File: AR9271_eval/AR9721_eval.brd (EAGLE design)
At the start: 160 x 100 mm, 125 parts, among them J1 UJ2-MIBH2-4-SMT-TR, J3 HTST-110-01-XX-DV, J7 132134-15, J8 132134-15, U1 U-ATHEROS-AR9271, U2 AT24C04C-XHM-T, U3 LT3080EQPBF, U4 LT3080EQPBF, U5 LT3080EQPBF, U6 LT3080EQPBF, Y1 ECS-400-10-36-CKY-TR

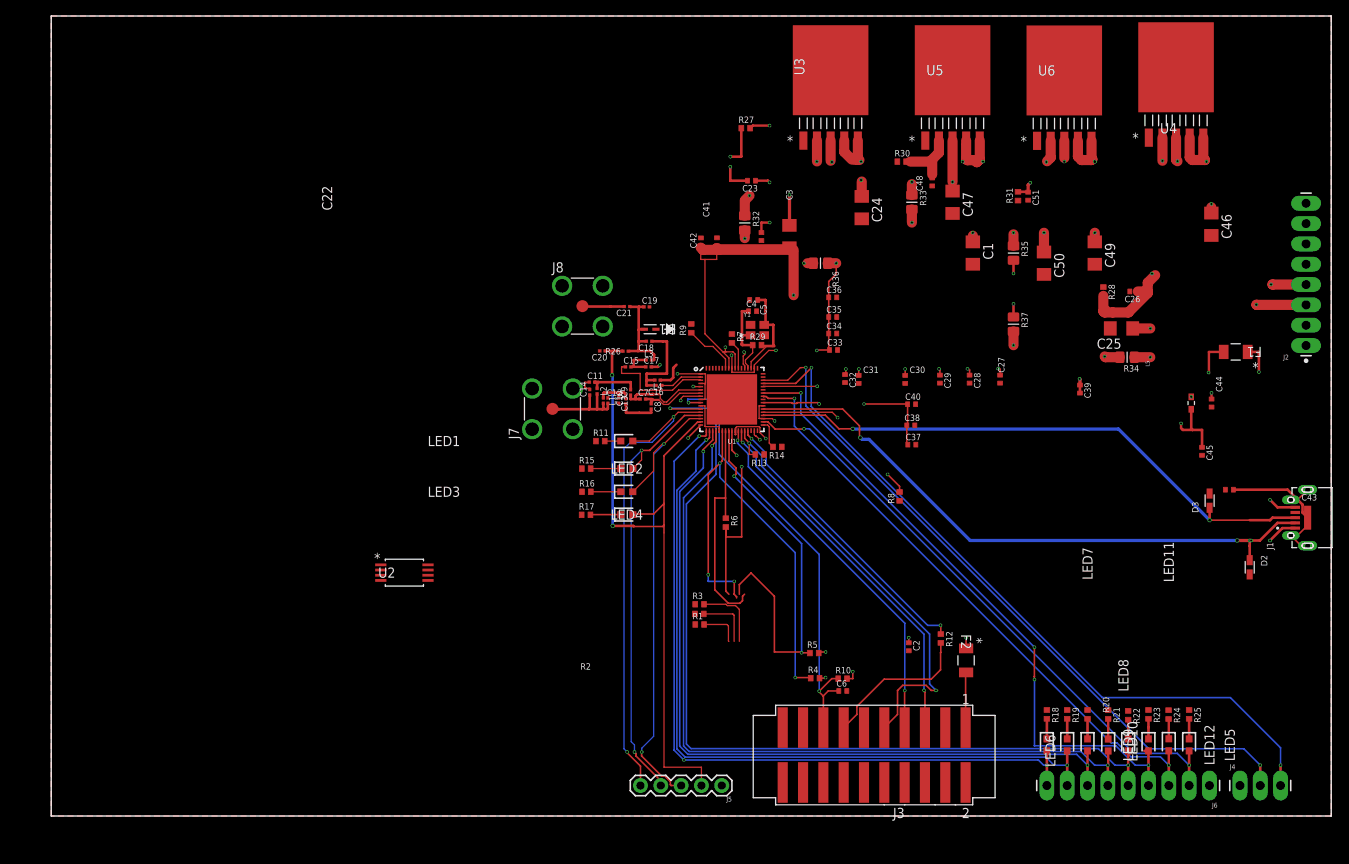
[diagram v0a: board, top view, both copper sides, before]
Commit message: Add files via upload
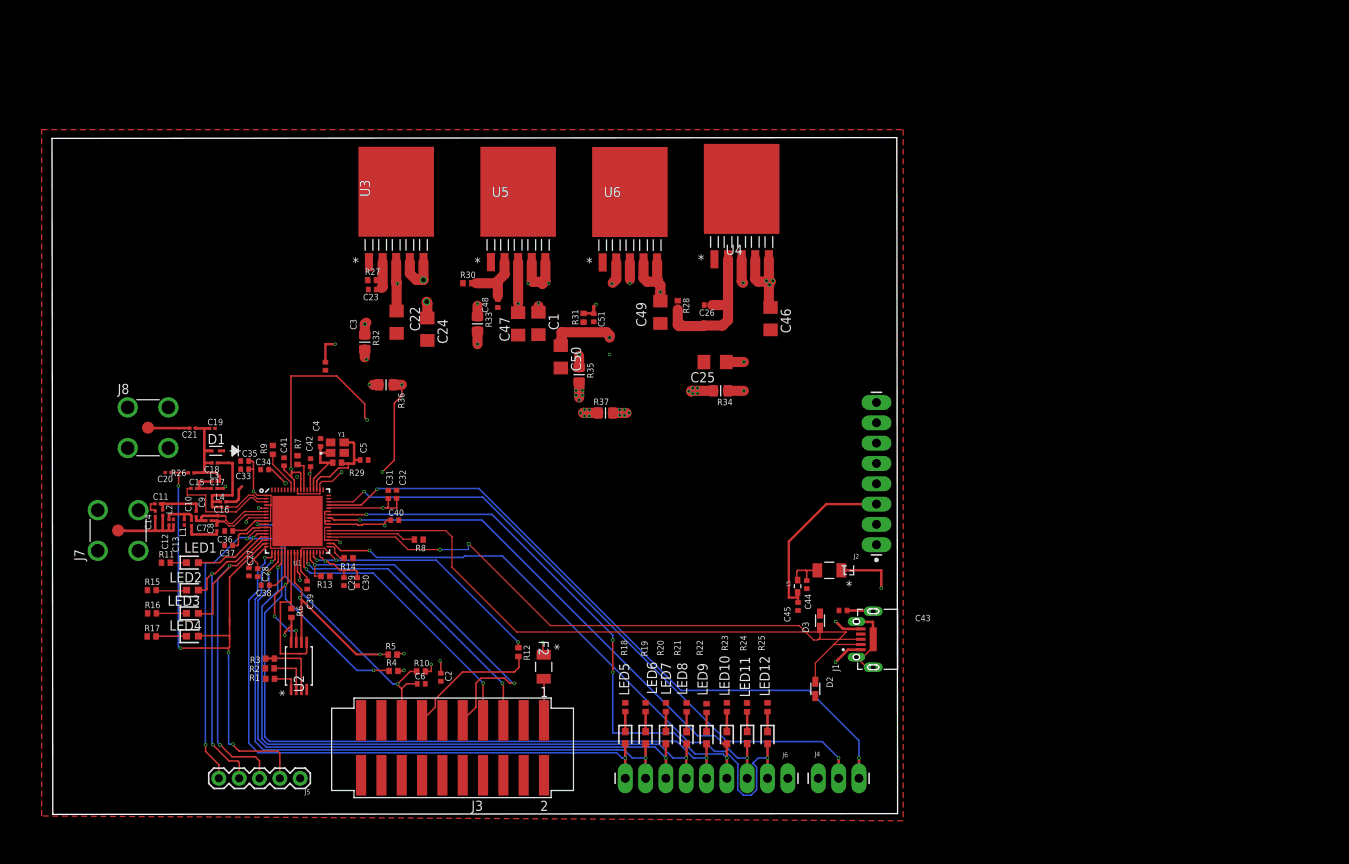
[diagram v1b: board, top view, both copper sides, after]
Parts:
- moved C39 99.7 mm to (32.0, 28.9)
- moved C27 96.9 mm to (24.7, 30.5)
- moved C28 92.2 mm to (25.8, 30.4)
- moved C37 86.3 mm to (22.2, 33.8), turned to 180 degrees
- moved C38 83.1 mm to (26.8, 28.8), turned to 180 degrees
- moved C36 80.9 mm to (22.2, 35.6), turned to 180 degrees
- moved C29 78.7 mm to (36.6, 29.3)
- moved C35 75.7 mm to (24.2, 44.4), turned to 180 degrees
- moved C33 75.1 mm to (24.2, 43.4), turned to 180 degrees
- moved C30 73.0 mm to (38.2, 29.3)
- moved C34 73.0 mm to (26.7, 43.3), turned to 180 degrees
- moved C40 66.2 mm to (43.0, 37.0)
- moved C50 61.5 mm to (63.7, 57.4)
- moved C41 60.7 mm to (29.1, 44.3)
- moved C31 60.5 mm to (42.1, 40.2), turned to 90 degrees
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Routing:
- net 3V3_D: track 202.7 -> 101.1 mm, vias 22 -> 15
- net LDO_IN: track 141.5 -> 90.0 mm, vias 11 -> 6
- net 1V2_A: track 91.9 -> 41.2 mm, vias 5 -> 3
- net N$25: track 53.2 -> 21.0 mm, vias 2 -> 0
- net N$3: track 57.8 -> 32.4 mm
- net GPIO11: track 114.3 -> 94.0 mm
- net N$23: track 23.2 -> 3.28 mm, vias 3 -> 0
- net RST_L: track 57.8 -> 41.0 mm
- net GPIO6: track 95.5 -> 78.8 mm
- net GPIO8: track 99.5 -> 82.7 mm
- net GPIO7: track 97.5 -> 80.7 mm
- net SWCOM1: track 55.9 -> 39.6 mm
- net GPIO5: track 93.7 -> 77.7 mm, vias 3 -> 2
- net SWCOM0: track 61.1 -> 45.1 mm
- net SWCOM2: track 60.7 -> 46.0 mm
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- removed copper zone on layer 15, net N$23
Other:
- board size 160 x 100 mm -> 105.7 x 84.6 mm

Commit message: Add files via upload
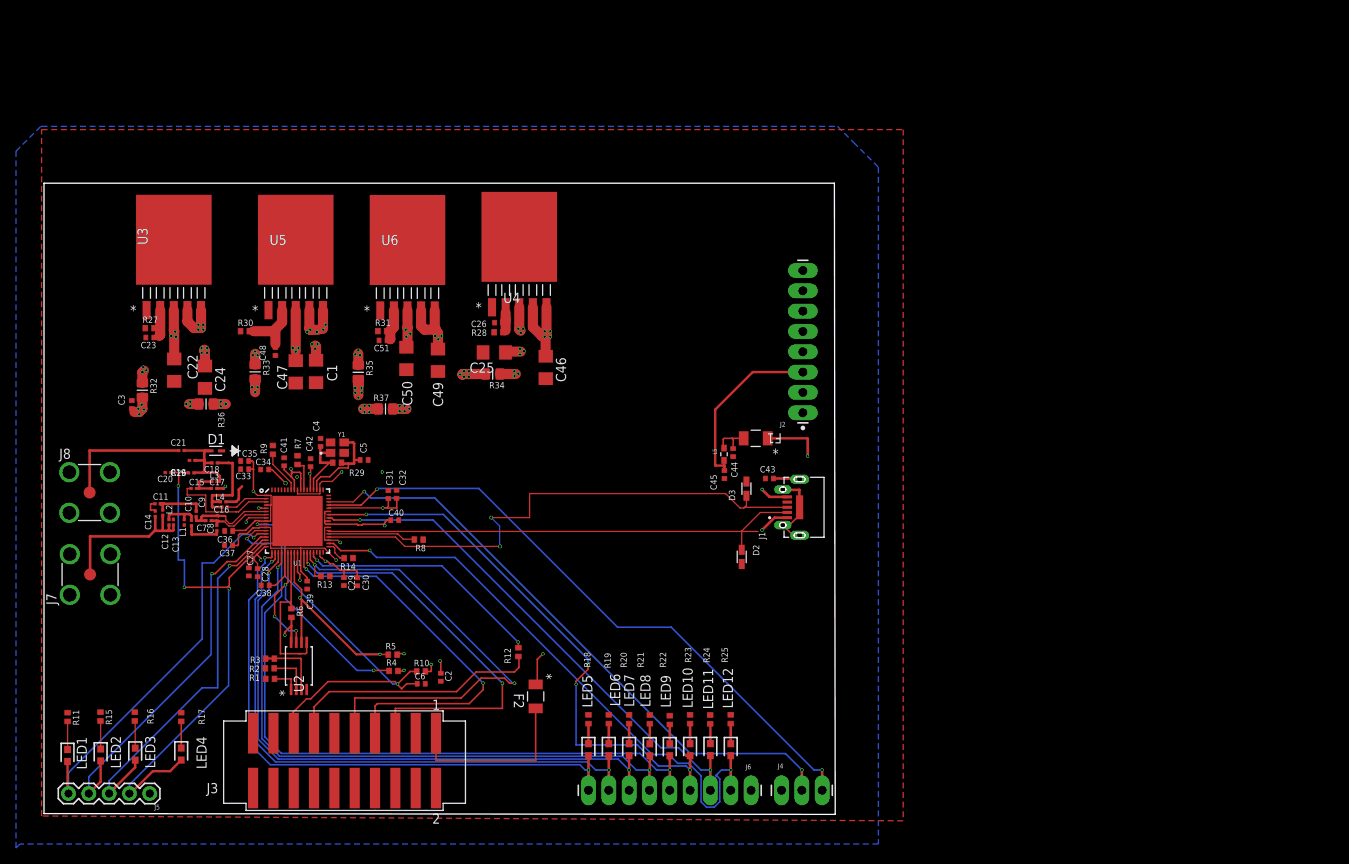
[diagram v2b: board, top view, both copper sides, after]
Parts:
- moved C46 28.8 mm to (61.8, 56.1)
- moved LED1 28.7 mm to (2.04, 7.56), turned to 270 degrees
- moved R34 28.6 mm to (55.2, 55.2)
- moved C22 28.4 mm to (15.4, 55.7)
- moved U4 28.4 mm to (58.5, 72.4)
- moved U6 28.4 mm to (44.5, 72.0)
- moved C23 28.4 mm to (12.3, 59.8)
- moved C47 28.4 mm to (30.6, 55.5)
- moved C48 28.4 mm to (28.0, 58.1)
- moved R33 28.4 mm to (25.5, 55.5)
- moved U5 28.4 mm to (30.6, 72.0)
- moved C1 28.4 mm to (33.1, 55.6)
- moved C24 28.4 mm to (19.2, 54.8)
- moved C49 28.4 mm to (48.3, 57.0)
- moved R27 28.4 mm to (12.3, 61.0)
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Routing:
- net LDO_IN: track 90.0 -> 122.6 mm, vias 6 -> 23
- net 1V2_D: track 90.0 -> 66.1 mm, vias 2 -> 12
- net USB_DM: track 83.4 -> 62.8 mm
- net N$32: track 5.22 -> 22.4 mm
- net N$25: track 21.0 -> 4.03 mm
- net 1V2_A: track 41.2 -> 24.9 mm, vias 3 -> 12
- net TDO: track 16.9 -> 32.4 mm
- net TCK: track 45.9 -> 60.9 mm
- net TDI: track 36.7 -> 51.6 mm
- net TMS: track 34.9 -> 48.8 mm
- net RST_L: track 41.0 -> 54.4 mm
- net 3V3_D: track 101.1 -> 114.1 mm, vias 15 -> 20
- net N$47: track 26.2 -> 14.2 mm, vias 4 -> 6
- net RCV_IN: track 5.29 -> 16.4 mm
- net N$37: track 22.0 -> 13.5 mm, vias 3 -> 9
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- added copper zone on layer 16, net GND
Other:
- board size 105.7 x 84.6 mm -> 98.9 x 78.9 mm

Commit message: Add files via upload
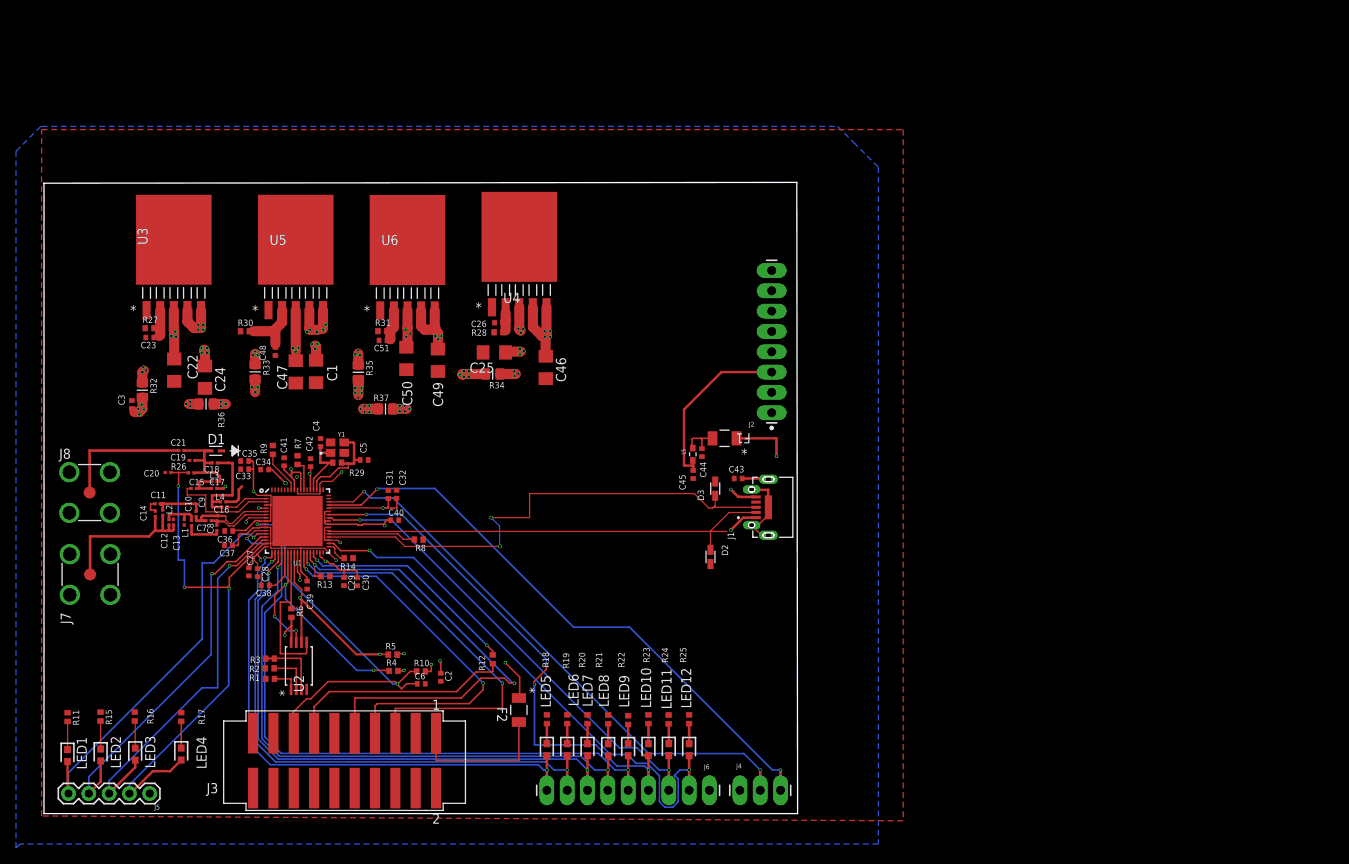
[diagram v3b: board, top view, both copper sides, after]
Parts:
- moved J4 5.20 mm to (86.1, 3.21)
- moved J6 5.20 mm to (82.3, 3.21)
- moved LED10 5.20 mm to (74.7, 8.29)
- moved LED11 5.20 mm to (77.2, 8.30)
- moved LED12 5.20 mm to (79.7, 8.29)
- moved LED6 5.20 mm to (64.5, 8.29)
- moved LED8 5.20 mm to (69.6, 8.28)
- moved R19 5.20 mm to (64.5, 12.1)
- moved R21 5.20 mm to (69.6, 12.1)
- moved R23 5.20 mm to (74.7, 12.1)
- moved R24 5.20 mm to (77.2, 12.1)
- moved R25 5.20 mm to (79.7, 12.1)
- moved LED5 5.20 mm to (62.0, 8.29)
- moved R18 5.20 mm to (62.0, 12.1)
- moved LED7 5.20 mm to (67.0, 8.29)
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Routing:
- net GPIO9: track 79.7 -> 74.5 mm
- net GPIO8: track 78.7 -> 73.5 mm
- net GPIO13: track 71.7 -> 66.5 mm
- net GPIO10: track 76.7 -> 71.5 mm
- net GPIO14: track 65.1 -> 59.9 mm
- net GPIO7: track 76.7 -> 71.5 mm
- net GPIO6: track 74.8 -> 69.6 mm
- net GPIO5: track 73.7 -> 68.5 mm
- net GPIO15: track 74.9 -> 69.7 mm
- net GPIO11: track 89.6 -> 84.4 mm
- net 3V3_A: track 63.9 -> 58.8 mm, vias 11 -> 10
- net TDO: track 32.4 -> 28.4 mm
- net USB_DM: track 62.8 -> 58.9 mm
- net USB_DP: track 68.3 -> 64.4 mm
- net LDO_IN: track 122.6 -> 118.7 mm
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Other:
- board size 98.9 x 78.9 mm -> 94.2 x 78.9 mm
